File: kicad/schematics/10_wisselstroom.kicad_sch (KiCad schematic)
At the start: 0 parts

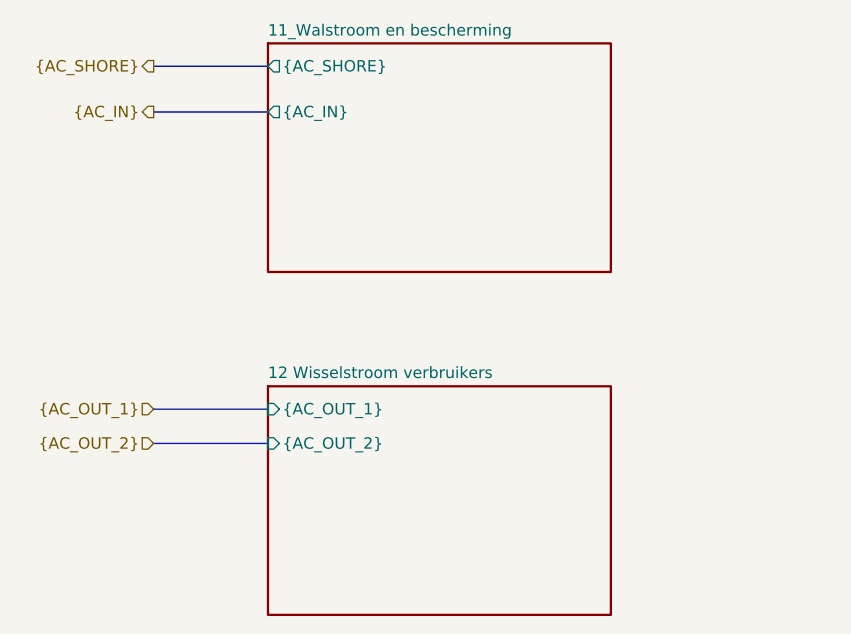
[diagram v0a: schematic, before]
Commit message: Schema's
00 toplevel stabiel
10 wisselstroom met subbladen stabiel
15 energieconversie stabiel
31 motor kern stabiel
32 motor sensoren stabiel
50 sensoren stabiel
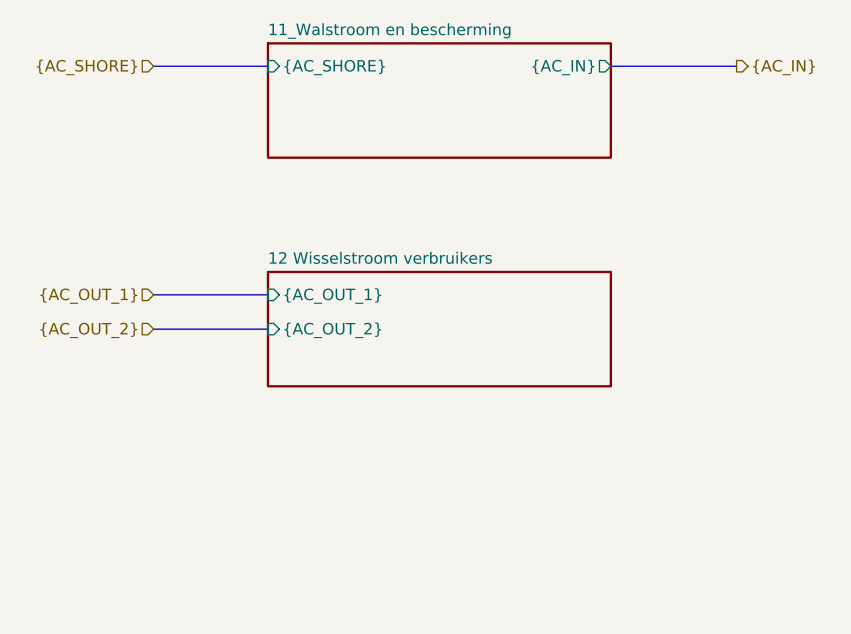
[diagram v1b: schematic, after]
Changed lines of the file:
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@@
 	(bus
 		(pts
-			(xy 76.2 78.74) (xy 88.9 78.74)
+			(xy 76.2 66.04) (xy 88.9 66.04)
 		)
 		(stroke
@@
 	(bus
 		(pts
-			(xy 76.2 45.72) (xy 88.9 45.72)
+			(xy 127 40.64) (xy 140.97 40.64)
 		)
 		(stroke
@@
 	(bus
 		(pts
-			(xy 76.2 82.55) (xy 88.9 82.55)
+			(xy 76.2 69.85) (xy 88.9 69.85)
 		)
 		(stroke
@@
 	)
 	(hierarchical_label "{AC_SHORE}"
-		(shape output)
+		(shape input)
 		(at 76.2 40.64 180)
 		(effects
@@
 	(hierarchical_label "{AC_OUT_1}"
 		(shape input)
-		(at 76.2 78.74 180)
+		(at 76.2 66.04 180)
 		(effects
 			(font
@@
 	(hierarchical_label "{AC_IN}"
 		(shape output)
-		(at 76.2 45.72 180)
+		(at 140.97 40.64 0)
 		(effects
 			(font
 				(size 1.27 1.27)
 			)
-			(justify right)
+			(justify left)
 		)
 	)
 	(hierarchical_label "{AC_OUT_2}"
 		(shape input)
-		(at 76.2 82.55 180)
+		(at 76.2 69.85 180)
 		(effects
 			(font
@@
 	(sheet
 		(at 88.9 38.1)
-		(size 38.1 25.4)
+		(size 38.1 12.7)
 		(exclude_from_sim no)
 		(in_bom yes)
@@
 		)
 		(property "Sheetname" "11_Walstroom en bescherming"
-			(at 88.9 37.3884 0)
+			(at 88.9 37.3376 0)
 			(show_name no)
 			(do_not_autoplace no)
@@
 		)
 		(property "Sheetfile" "11_walstroom_en_bescherming.kicad_sch"
-			(at 88.9 64.0846 0)
+			(at 88.9 51.4354 0)
 			(hide yes)
 			(show_name no)
@@
 			)
 		)
-		(pin "{AC_SHORE}" output
+		(pin "{AC_SHORE}" input
 			(at 88.9 40.64 180)
 			(effects
@@
 		)
 		(pin "{AC_IN}" output
-			(at 88.9 45.72 180)
+			(at 127 40.64 0)
 			(effects
 				(font
 					(size 1.27 1.27)
 				)
-				(justify left)
+				(justify right)
 			)
 		)
@@
 	)
 	(sheet
-		(at 88.9 76.2)
-		(size 38.1 25.4)
+		(at 88.9 63.5)
+		(size 38.1 12.7)
 		(exclude_from_sim no)
 		(in_bom yes)
@@
 		)
 		(property "Sheetname" "12 Wisselstroom verbruikers"
-			(at 88.9 75.4376 0)
+			(at 88.9 62.7376 0)
 			(show_name no)
 			(do_not_autoplace no)
@@
 		)
 		(property "Sheetfile" "12_ac_verbruikers.kicad_sch"
-			(at 88.9 102.2354 0)
+			(at 88.9 76.8354 0)
 			(hide yes)
 			(show_name no)
@@
 		)
 		(pin "{AC_OUT_1}" input
-			(at 88.9 78.74 180)
+			(at 88.9 66.04 180)
 			(effects
 				(font
@@
 		)
 		(pin "{AC_OUT_2}" input
-			(at 88.9 82.55 180)
+			(at 88.9 69.85 180)
 			(effects
 				(font
